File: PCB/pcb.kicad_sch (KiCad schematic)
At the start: 7 parts, among them SW1 SW_Push, SW2 SW_Push, SW3 SW_Push, SW4 SW_Push, U1 XIAO-RP2040-DIP

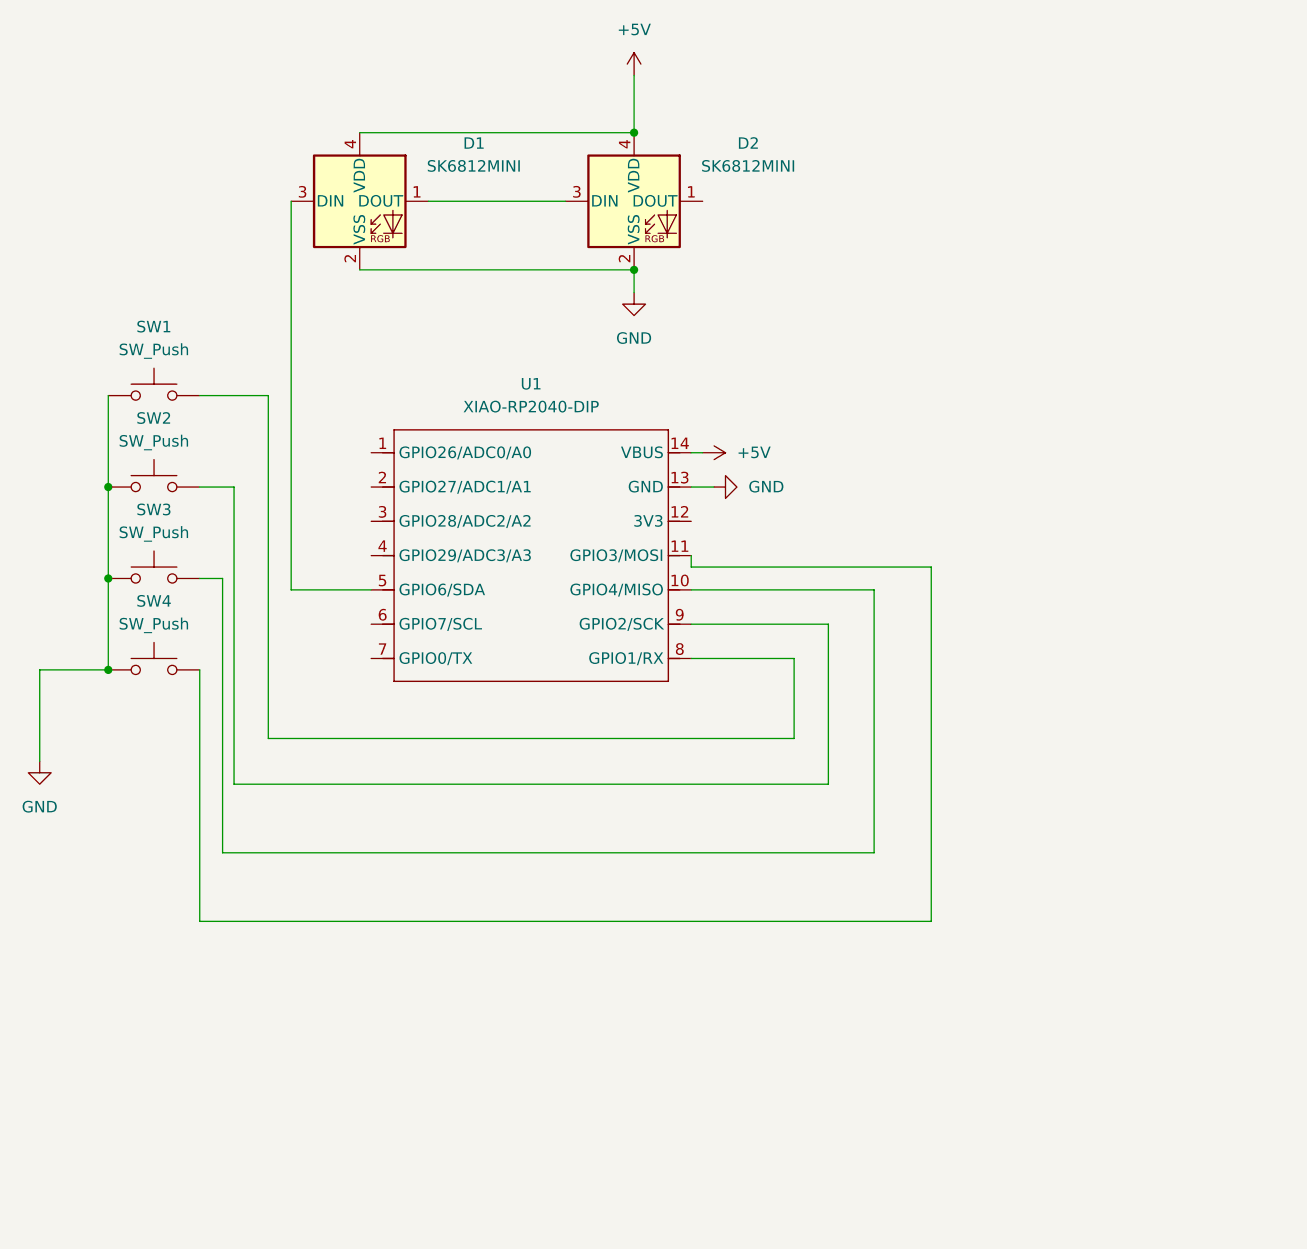
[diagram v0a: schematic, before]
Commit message: Dodanie nowych plików i zmian
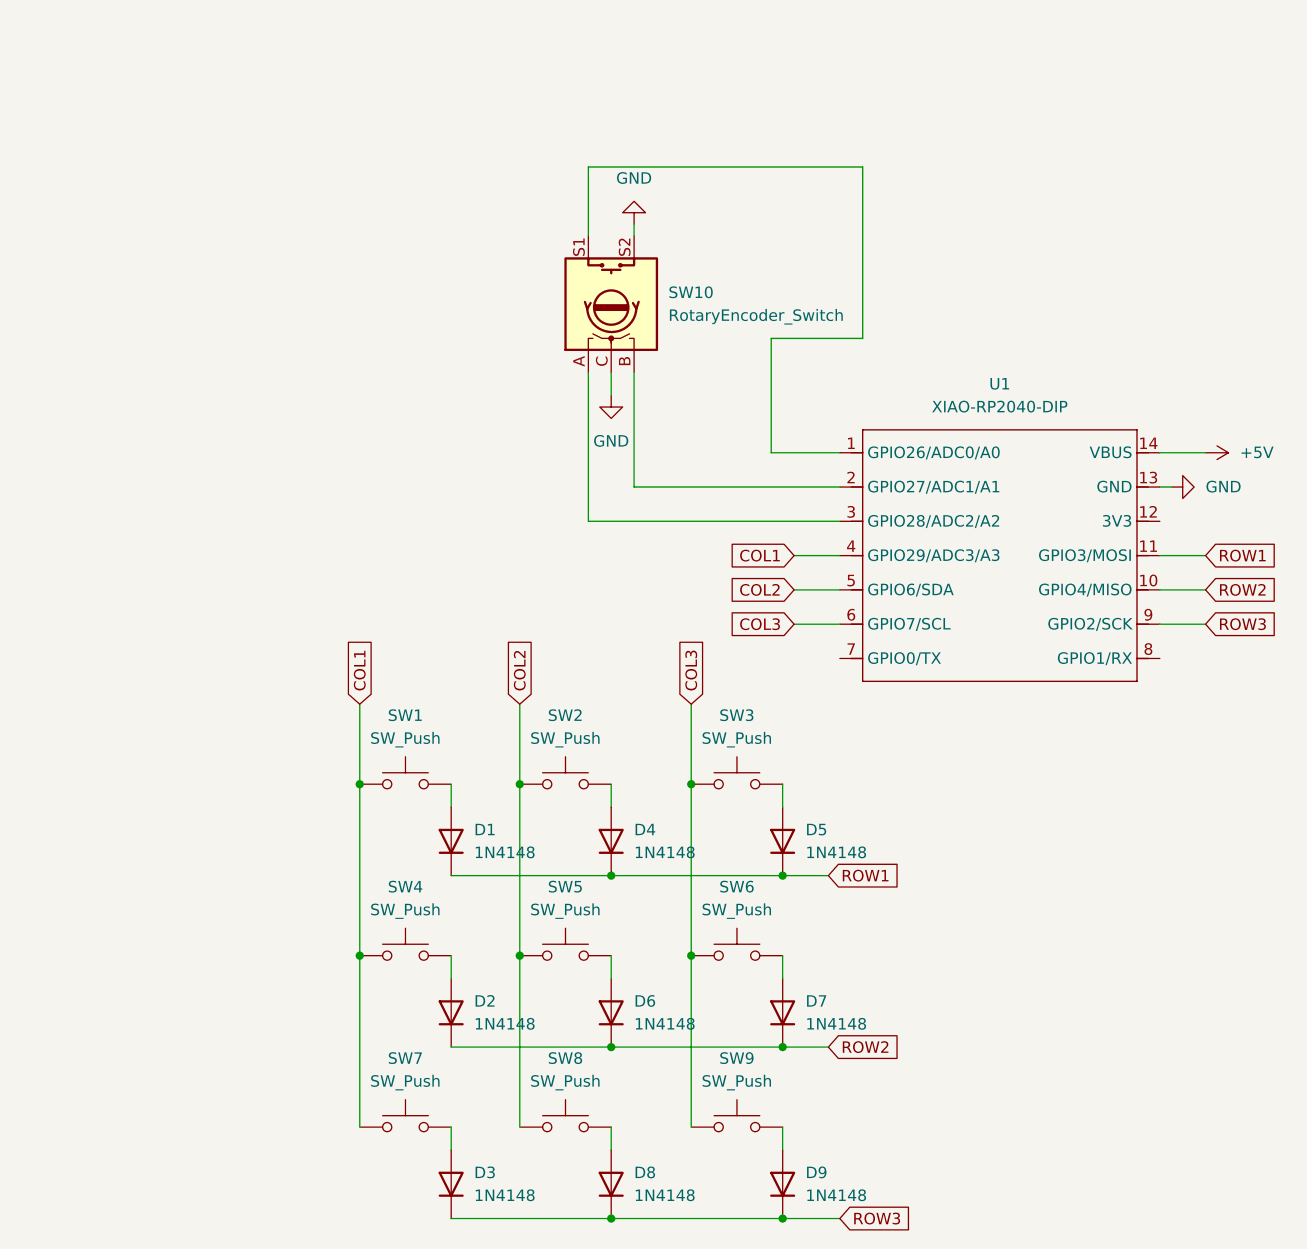
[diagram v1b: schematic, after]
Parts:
- removed D1, D2: SK6812MINI, LED_SMD:LED_SK6812MINI_PLCC4_3.5x3.5mm_P1.75mm, symbol LED:SK6812MINI
- added D1, D2, D3, D4, D5, D6, D7, D8, D9: 1N4148, Diode_THT:D_DO-35_SOD27_P7.62mm_Horizontal, symbol Diode:1N4148
- added SW10: RotaryEncoder_Switch, Rotary_Encoder:RotaryEncoder_Alps_EC11E-Switch_Vertical_H20mm_CircularMountingHoles, symbol Device:RotaryEncoder_Switch
- added SW5, SW6, SW7, SW8, SW9: SW_Push, Button_Switch_Keyboard:SW_Cherry_MX_1.00u_PCB, symbol Switch:SW_Push
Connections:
- net GND: now also SW10.C, SW10.S2; no longer SW1.1, SW2.1, SW3.1, SW4.1
- net COL2: now reaches U1.5 (GPIO6/SDA)
- net COL2: now also SW2.1, SW5.1, SW8.1
- net at SW2.2: now also D4.2 (A); no longer U1.9 (GPIO2/SCK)
- net at SW4.2: now also D2.2 (A); no longer U1.11 (GPIO3/MOSI)
- net at SW3.2: now also D5.2 (A); no longer U1.10 (GPIO4/MISO)
- net at SW1.2: now also D1.2 (A); no longer U1.8 (GPIO1/RX)
- net at U1.1 (GPIO26/ADC0/A0): now also SW10.S1
- net at U1.2 (GPIO27/ADC1/A1): now also SW10.B
- net at U1.3 (GPIO28/ADC2/A2): now also SW10.A
- net COL1: now reaches U1.4 (GPIO29/ADC3/A3)
- net COL1: now also SW1.1, SW4.1, SW7.1
- net COL3: now reaches U1.6 (GPIO7/SCL)
- net COL3: now also SW3.1, SW6.1, SW9.1
- new net: D9.2 (A), SW9.2
- new net: D8.2 (A), SW8.2
- new net: D3.2 (A), SW7.2
- new net: D6.2 (A), SW5.2
- new net: D7.2 (A), SW6.2
- new net ROW1: D1.1 (K), D4.1 (K), D5.1 (K), U1.11 (GPIO3/MOSI)
- new net ROW2: D2.1 (K), D6.1 (K), D7.1 (K), U1.10 (GPIO4/MISO)
- new net ROW3: D3.1 (K), D8.1 (K), D9.1 (K), U1.9 (GPIO2/SCK)
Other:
- moved on the sheet: U1
